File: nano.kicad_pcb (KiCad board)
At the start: 2 copper layers, 183.7 x 126.7 mm, 25 parts, among them M1 Motor_DC, Q1 BP103, Q2 NPN, Q3 NPN, SW1 SW_Push

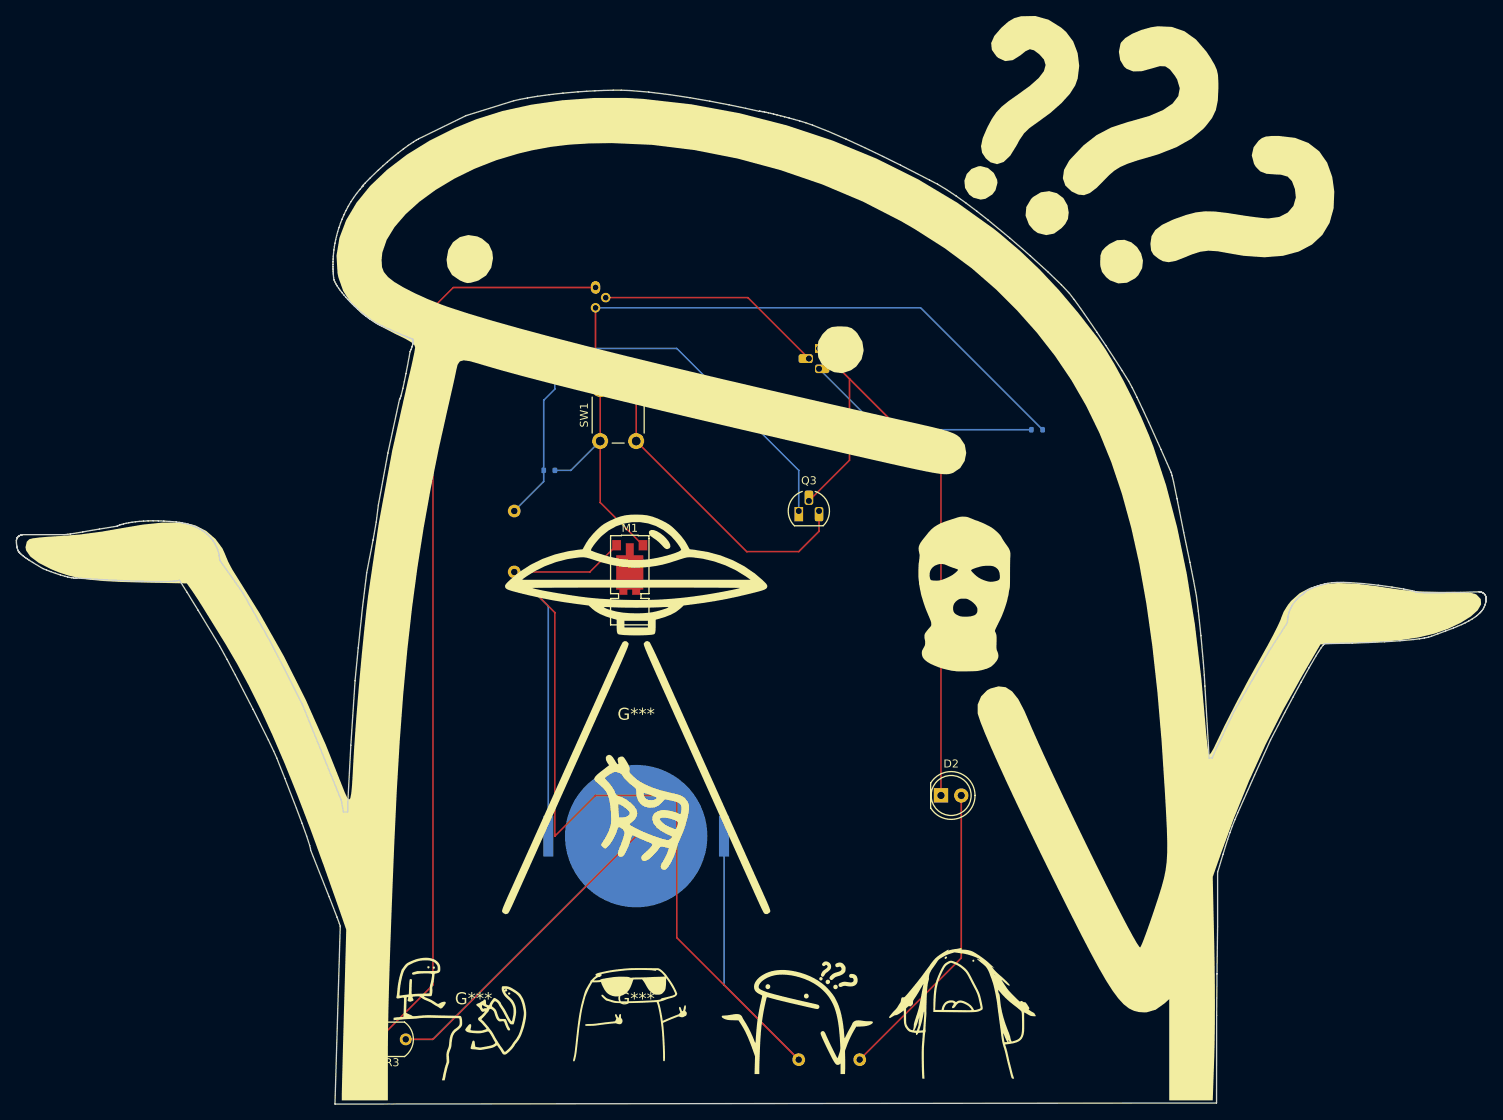
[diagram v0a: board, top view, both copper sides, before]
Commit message: the last
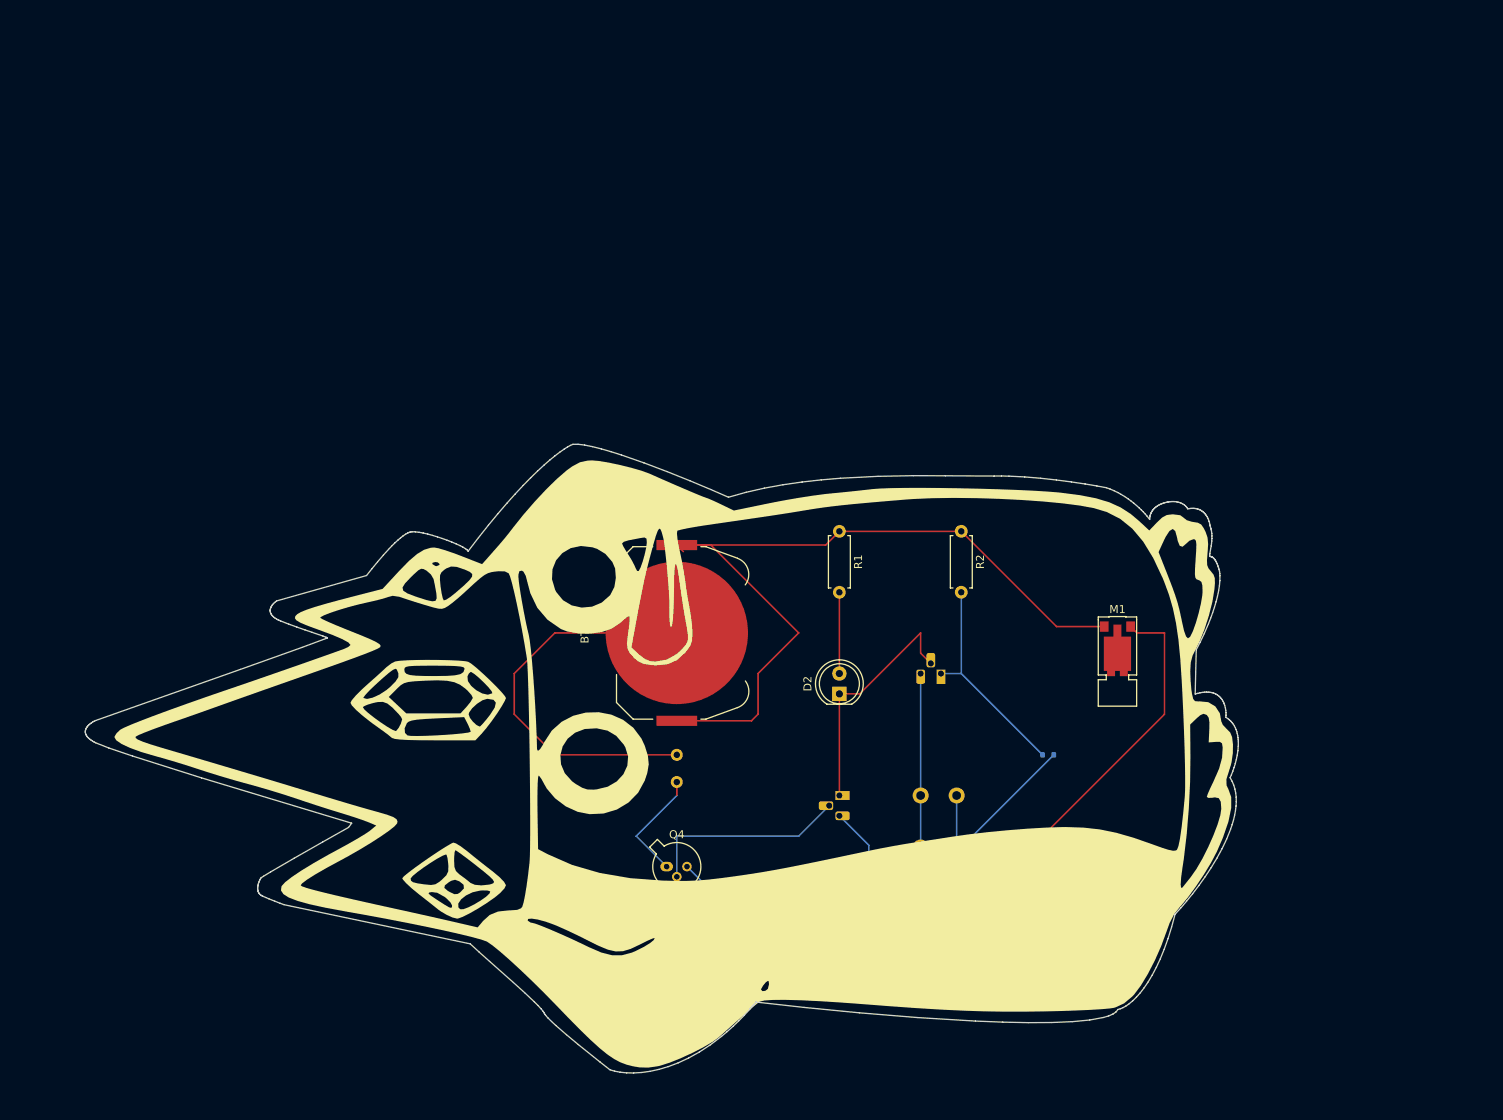
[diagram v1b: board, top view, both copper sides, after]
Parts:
- removed the G*** at (86.4, 162.6) (x2)
- removed the G*** at (91.4, 91.4)
- removed the G*** at (132.1, 147.3)
- removed the G*** at (66.0, 162.6) (x2)
- removed the G*** at (127.0, 111.8)
- removed the G*** at (102.7, 84.5)
- removed the G*** at (86.4, 127.0)
- removed the G*** at (127.0, 162.6)
- removed the G*** at (127.4, 76.2)
- removed the G*** at (127.0, 101.6)
- removed Q1: BP103, Package_TO_SOT_THT:TO-18-3_Lens
- removed `: LOGO, LOGO
- added G***: LOGO, LOGO, F.Cu at (96.5, 132.1)
- added G***: LOGO, LOGO, B.Cu at (96.5, 132.1)
- added Q4: BP103, Package_TO_SOT_THT:TO-18-3_Lens, F.Cu at (90.2, 146.1)
- BT1, R1, R2: moved to F.Cu
- Q3, R3, SW1: moved to B.Cu
- moved D3 71.8 mm to (137.9, 132.1)
- moved SW1 67.6 mm to (126.4, 143.7)
- moved R1 66.2 mm to (111.8, 104.1), turned to -90 degrees
- moved M1 61.8 mm to (146.5, 120.4)
- moved D1 59.5 mm to (116.1, 147.3)
- moved R2 56.1 mm to (127.0, 104.1), turned to -90 degrees
- moved Q2 55.9 mm to (111.8, 137.2)
- moved R3 49.1 mm to (91.4, 132.1), turned to -90 degrees
- moved Q3 27.0 mm to (124.5, 121.9), turned to 180 degrees
- moved BT1 25.9 mm to (91.4, 116.8), turned to 90 degrees
- moved D2 18.0 mm to (111.8, 124.5), turned to 90 degrees
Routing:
- net Net-(Q4-E): track 115.6 -> 15.9 mm
- net Net-(BT1-+): track 172.6 -> 102.8 mm
- net Net-(D2-K): track 79.5 -> 30.4 mm
- net Net-(D3-A): track 64.3 -> 27.1 mm
- net Net-(BT1--): track 78.6 -> 49.9 mm
- net Net-(D2-A): track 38.3 -> 10.2 mm
- net Net-(D1-A): track 29.7 -> 9.14 mm
- net Net-(Q3-E): track 38.7 -> 21.7 mm
- net Net-(D1-K): track 101.5 -> 114.0 mm
- net Net-(Q2-B): track 28.6 -> 25.7 mm
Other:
- board size 183.7 x 126.7 mm -> 144.1 x 78.6 mm
